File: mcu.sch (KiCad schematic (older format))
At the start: 34 parts, among them J4 Conn_01x04_Male, Q34 NX7002AK, SW21 SW_Push, SW22 SW_Push, U4 USBUF, U5 STM32F411RCT6, U7 LTV-357T, Y1 8MHz

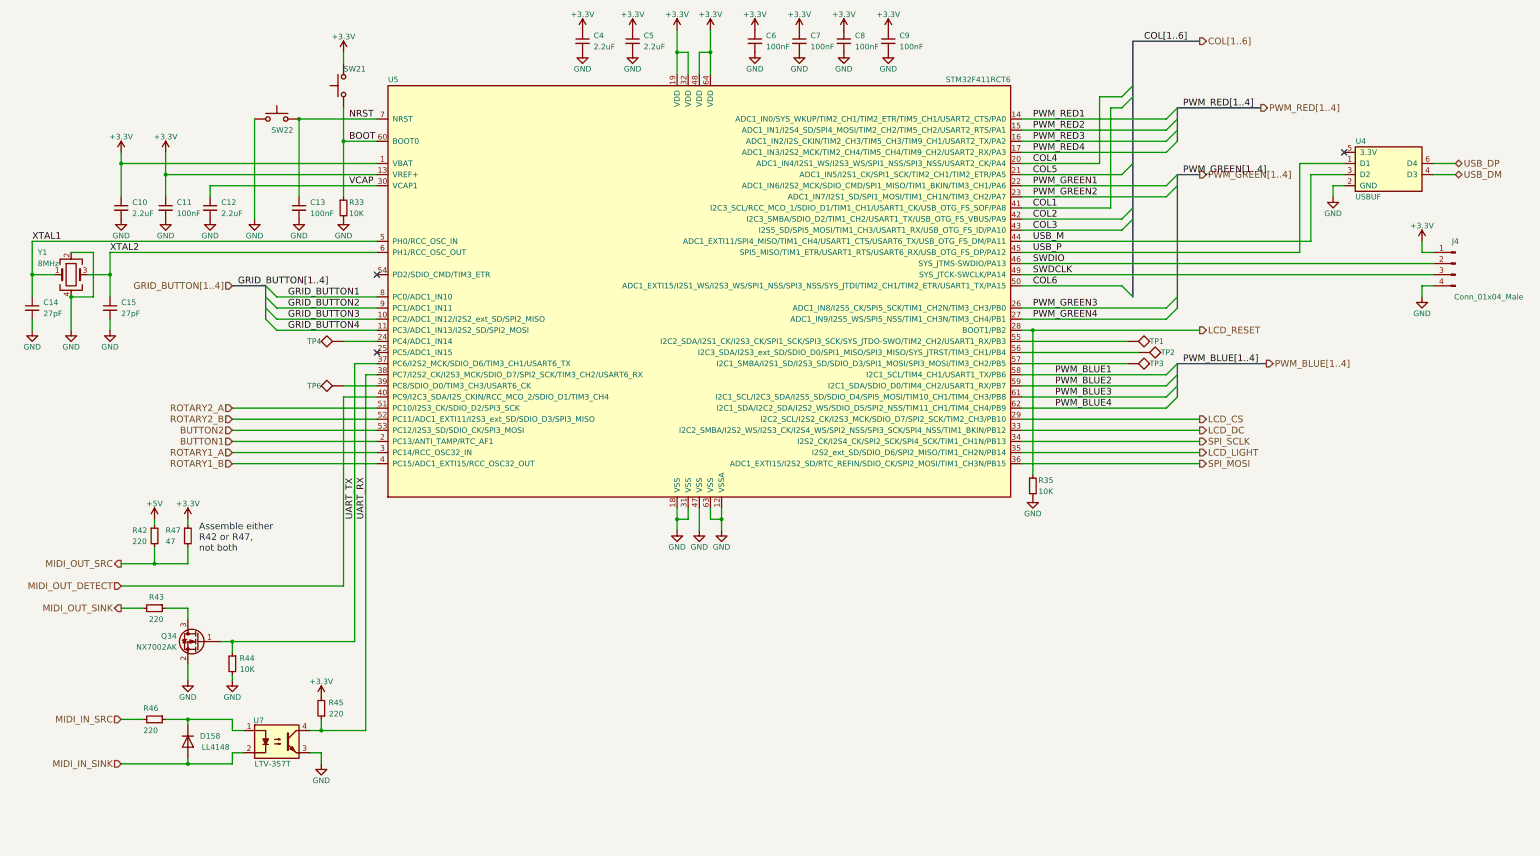
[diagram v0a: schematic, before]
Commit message: commiting before bulk led schematic symbol change
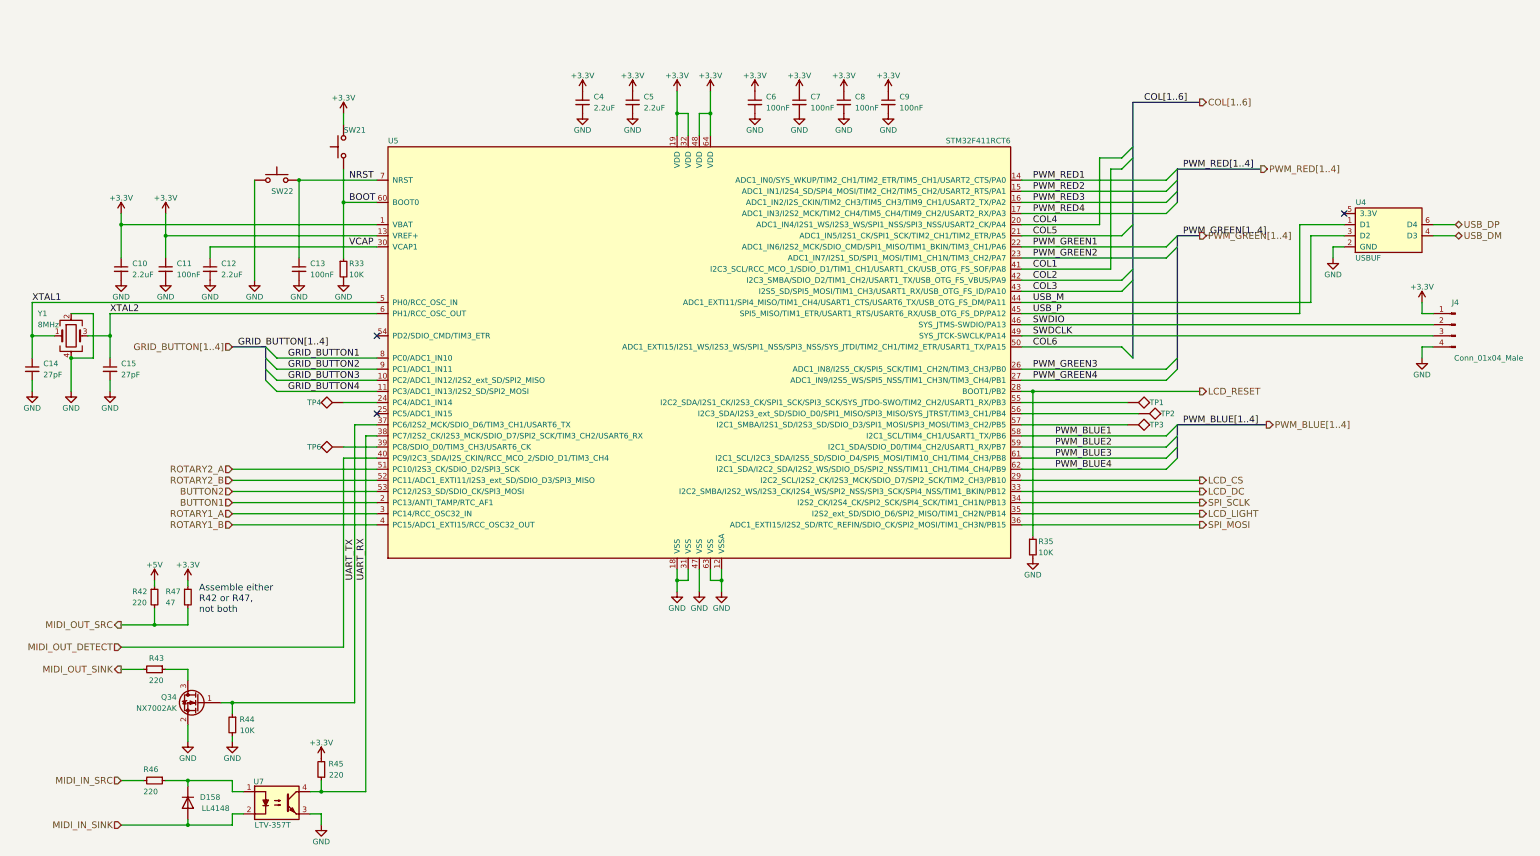
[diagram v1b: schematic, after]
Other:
- moved on the sheet: C10, C11, C12, C13, C14, C15, C4, C5, C6, C7, C8, C9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
